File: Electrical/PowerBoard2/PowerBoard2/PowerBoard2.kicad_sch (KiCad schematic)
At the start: 14 parts, among them J1 XT60PW-M, J2 XT60PW-M, J3 B4B-XH-A_LF__SN_, J5 XT60PW-M, U2 INA226AIDGSR, U3 USB-A-S-RA-TSMT

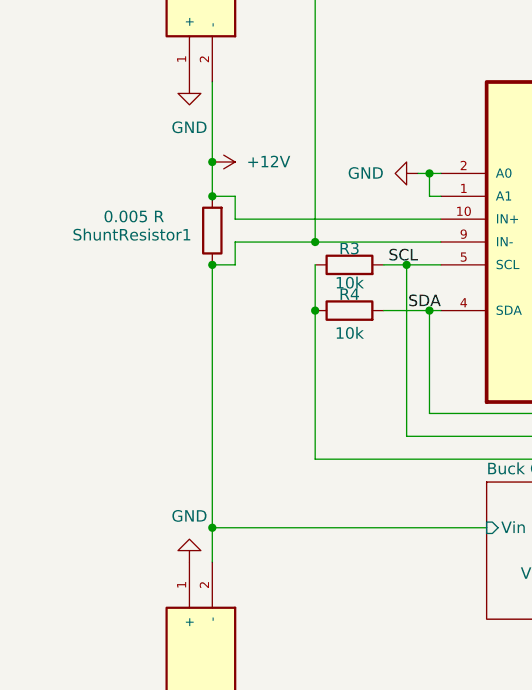
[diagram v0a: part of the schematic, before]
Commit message: shunt
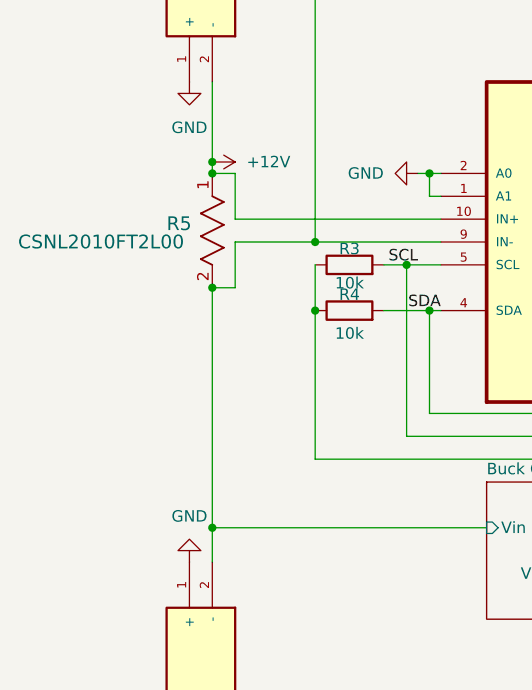
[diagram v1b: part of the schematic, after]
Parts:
- removed ShuntResistor1: 0.005 R, Resistor_SMD:R_2010_5025Metric_Pad1.40x2.65mm_HandSolder, symbol Device:R
- added R5: CSNL2010FT2L00, Shuntresistor:STA_CSNL2010&lessthan_=3_STP, symbol 2025-05-07_20-00-53:CSNL2010FT2L00
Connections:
- net +12V: now also R5.1
- net Buck Converter/Vin (12V): now also R5.2
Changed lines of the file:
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@@
-	)
-	(junction
-		(at 43.18 76.2)
-		(diameter 0)
-		(color 0 0 0 0)
 	)
 	(junction
@@
 	)
 	(junction
+		(at 43.18 73.66)
+		(diameter 0)
+		(color 0 0 0 0)
+	)
+	(junction
 		(at 135.89 160.02)
 		(diameter 0)
@@
 	)
 	(junction
-		(at 43.18 83.82)
-		(diameter 0)
-		(color 0 0 0 0)
-	)
-	(junction
 		(at 110.49 138.43)
 		(diameter 0)
@@
 		(color 0 0 0 0)
 	)
+	(junction
+		(at 43.18 86.36)
+		(diameter 0)
+		(color 0 0 0 0)
+	)
 	(no_connect
 		(at 99.06 168.91)
@@
 	(wire
 		(pts
-			(xy 45.72 76.2) (xy 43.18 76.2)
+			(xy 45.72 73.66) (xy 43.18 73.66)
 		)
 		(stroke
@@
 	(wire
 		(pts
-			(xy 43.18 83.82) (xy 45.72 83.82)
+			(xy 45.72 86.36) (xy 43.18 86.36)
 		)
 		(stroke
@@
 	(wire
 		(pts
-			(xy 45.72 83.82) (xy 45.72 81.28)
+			(xy 45.72 86.36) (xy 45.72 81.28)
 		)
 		(stroke
@@
 	(wire
 		(pts
-			(xy 43.18 83.82) (xy 43.18 113.03)
+			(xy 43.18 86.36) (xy 43.18 113.03)
 		)
 		(stroke
@@
 	(wire
 		(pts
-			(xy 43.18 72.39) (xy 43.18 76.2)
+			(xy 43.18 72.39) (xy 43.18 73.66)
 		)
 		(stroke
@@
 	(wire
 		(pts
-			(xy 45.72 78.74) (xy 45.72 76.2)
+			(xy 45.72 78.74) (xy 45.72 73.66)
 		)
 		(stroke
@@
 	)
 	(symbol
-		(lib_id "Device:R")
-		(at 43.18 80.01 180)
+		(lib_id "2025-05-07_20-00-53:CSNL2010FT2L00")
+		(at 43.18 73.66 270)
 		(unit 1)
 		(exclude_from_sim no)
@@
 		(on_board yes)
 		(dnp no)
-		(property "Reference" "ShuntResistor1"
-			(at 40.894 80.518 0)
-			(effects
-				(font
-					(size 1.27 1.27)
+		(property "Reference" "R5"
+			(at 38.1 79.248 90)
+			(effects
+				(font
+					(size 1.524 1.524)
 				)
 				(justify left)
 			)
 		)
-		(property "Value" "0.005 R"
-			(at 37.846 78.486 0)
-			(effects
-				(font
-					(size 1.27 1.27)
+		(property "Value" "CSNL2010FT2L00"
+			(at 21.59 81.2799 90)
+			(effects
+				(font
+					(size 1.524 1.524)
 				)
 				(justify left)
 			)
 		)
-		(property "Footprint" "Resistor_SMD:R_2010_5025Metric_Pad1.40x2.65mm_HandSolder"
-			(at 44.958 80.01 90)
-			(effects
-				(font
-					(size 1.27 1.27)
-				)
-				(hide yes)
-			)
-		)
-		(property "Datasheet" "~"
-			(at 43.18 80.01 0)
-			(effects
-				(font
-					(size 1.27 1.27)
-				)
-				(hide yes)
-			)
-		)
-		(property "Description" "Resistor"
-			(at 43.18 80.01 0)
-			(effects
-				(font
-					(size 1.27 1.27)
-				)
-				(hide yes)
-			)
+		(property "Footprint" "Shuntresistor:STA_CSNL2010&lessthan_=3_STP"
+			(at 43.18 73.66 0)
+			(effects
+				(font
+					(size 1.27 1.27)
+					(italic yes)
+				)
+				(hide yes)
+			)
+		)
+		(property "Datasheet" "CSNL2010FT2L00"
+			(at 43.18 73.66 0)
+			(effects
+				(font
+					(size 1.27 1.27)
+					(italic yes)
+				)
+				(hide yes)
+			)
+		)
+		(property "Description" ""
+			(at 43.18 73.66 0)
+			(effects
+				(font
+					(size 1.27 1.27)
+				)
+				(hide yes)
+			)
+		)
+		(pin "2"
 		)
 		(pin "1"
-		)
-		(pin "2"
 		)
 		(instances
 			(project ""
 				(path "/f95f296f-a4bf-4952-bdc7-66087a6cc347"
-					(reference "ShuntResistor1")
+					(reference "R5")
 					(unit 1)
 				)

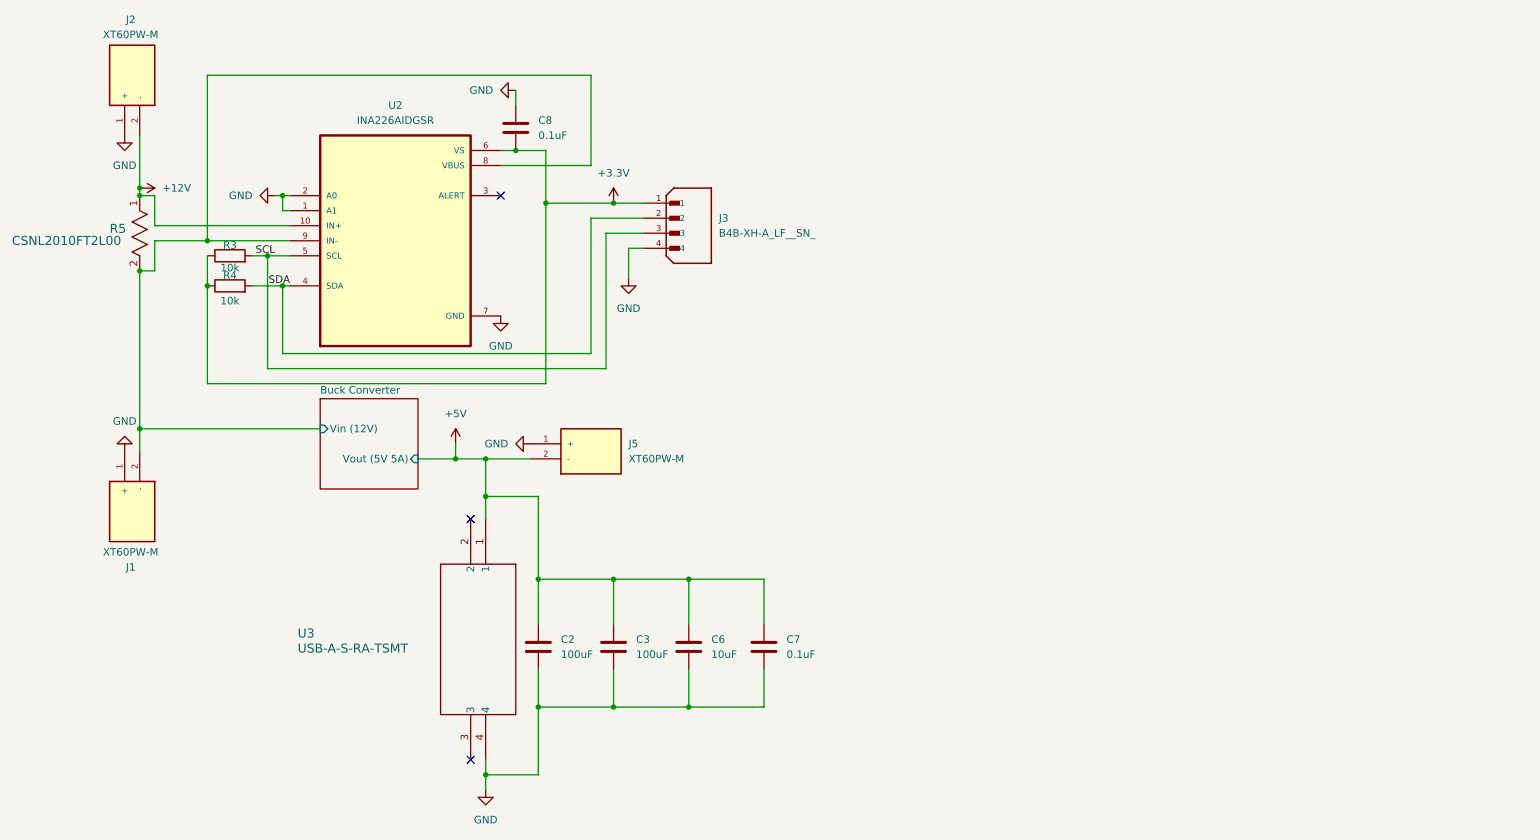
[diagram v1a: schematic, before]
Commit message: capacitors and opamps
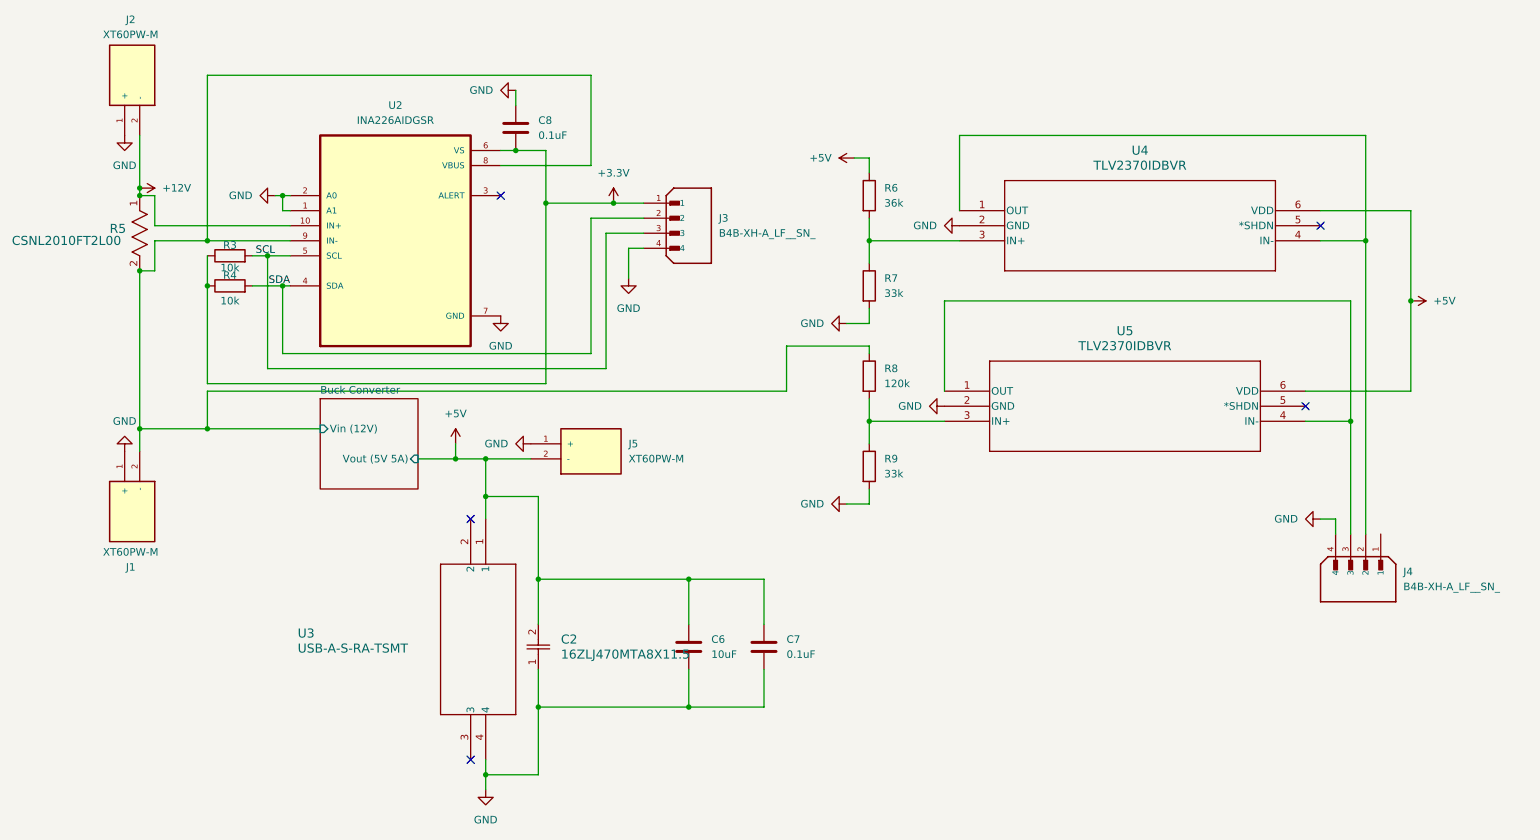
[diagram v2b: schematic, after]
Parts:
- removed C2, C3: 100uF, Capacitor_SMD:C_0805_2012Metric_Pad1.18x1.45mm_HandSolder, symbol Device:C
- added C2: 16ZLJ470MTA8X11.5, CAP_YX_8X11P5_RUB, symbol 2025-05-07_21-08-47:16ZLJ470MTA8X11.5
- added J4: B4B-XH-A_LF__SN_, B4B-XH-A_LF__SN_:JST_B4B-XH-A_LF__SN_, symbol B4B-XH-A_LF__SN_:B4B-XH-A_LF__SN_
- added R6: 36k, Resistor_SMD:R_0805_2012Metric_Pad1.20x1.40mm_HandSolder, symbol Device:R
- added R7, R9: 33k, Resistor_SMD:R_0805_2012Metric_Pad1.20x1.40mm_HandSolder, symbol Device:R
- added R8: 120k, Resistor_SMD:R_0805_2012Metric_Pad1.20x1.40mm_HandSolder, symbol Device:R
- added U4, U5: TLV2370IDBVR, DBV6, symbol 2025-02-22_17-10-12:TLV2370IDBVR
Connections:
- net +5V: now also C2.2, R6.1, U4.6 (VDD), U5.6 (VDD)
- net Buck Converter/Vin (12V): now also R8.1
- net GND: now also C2.1, J4.4, R7.2, R9.2, U4.2 (GND), U5.2 (GND)
- new net: J4.3, U5.1 (OUT), U5.4 (IN-)
- new net: R8.2, R9.1, U5.3 (IN+)
- new net: R6.2, R7.1, U4.3 (IN+)
- new net: J4.2, U4.1 (OUT), U4.4 (IN-)
- no-connect marks 3 -> 5
